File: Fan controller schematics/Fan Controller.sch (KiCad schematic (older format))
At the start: 6 parts, among them IC1 ATMEGA328-P, SW1 ROTARY_ENCODER, Y1 16MHz

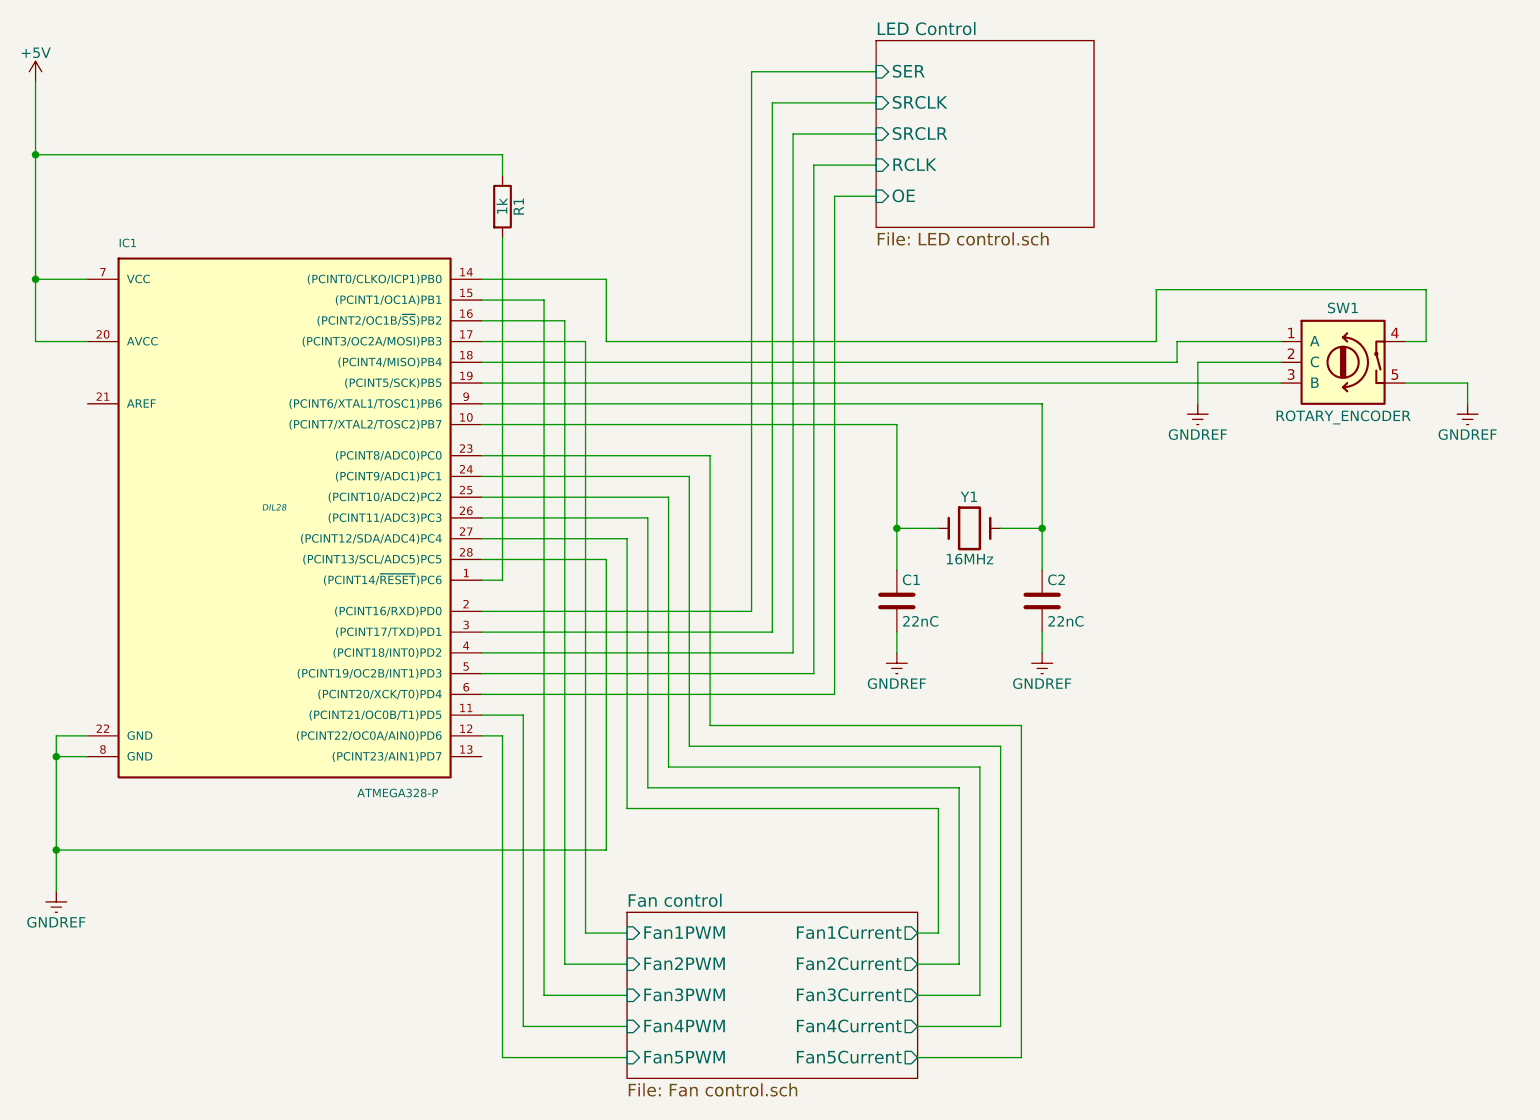
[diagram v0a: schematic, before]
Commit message: Small routing change
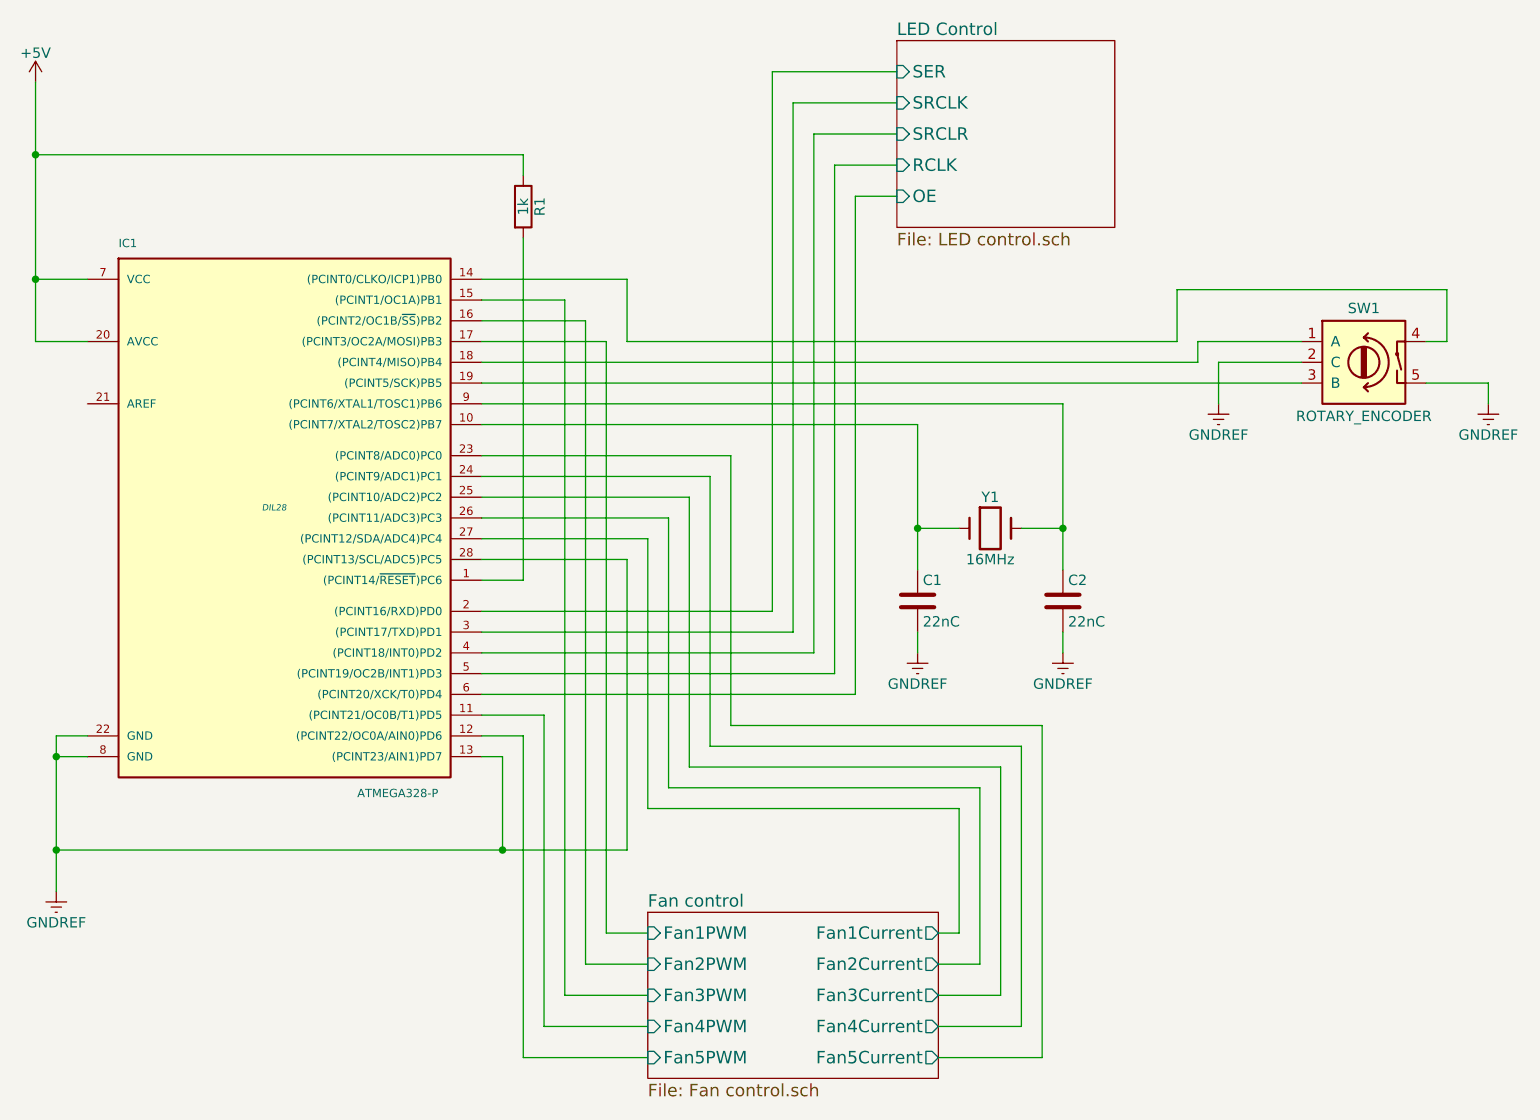
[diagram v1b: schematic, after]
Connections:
- net GNDREF: now also IC1.13 ((PCINT23/AIN1)PD7)
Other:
- moved on the sheet: C1, C2, R1, SW1, Y1
